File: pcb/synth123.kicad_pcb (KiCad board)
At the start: 2 copper layers, 100 x 50 mm, 29 parts, among them IC1 ATTINY4313, IC2 PC817, IC3 DAC, K1 STEREO/MONO, P1 POWER, P2 MIDI_IN, P3 ISP, P4 AUDIO_OUT, U1 7805, X1 20MHz

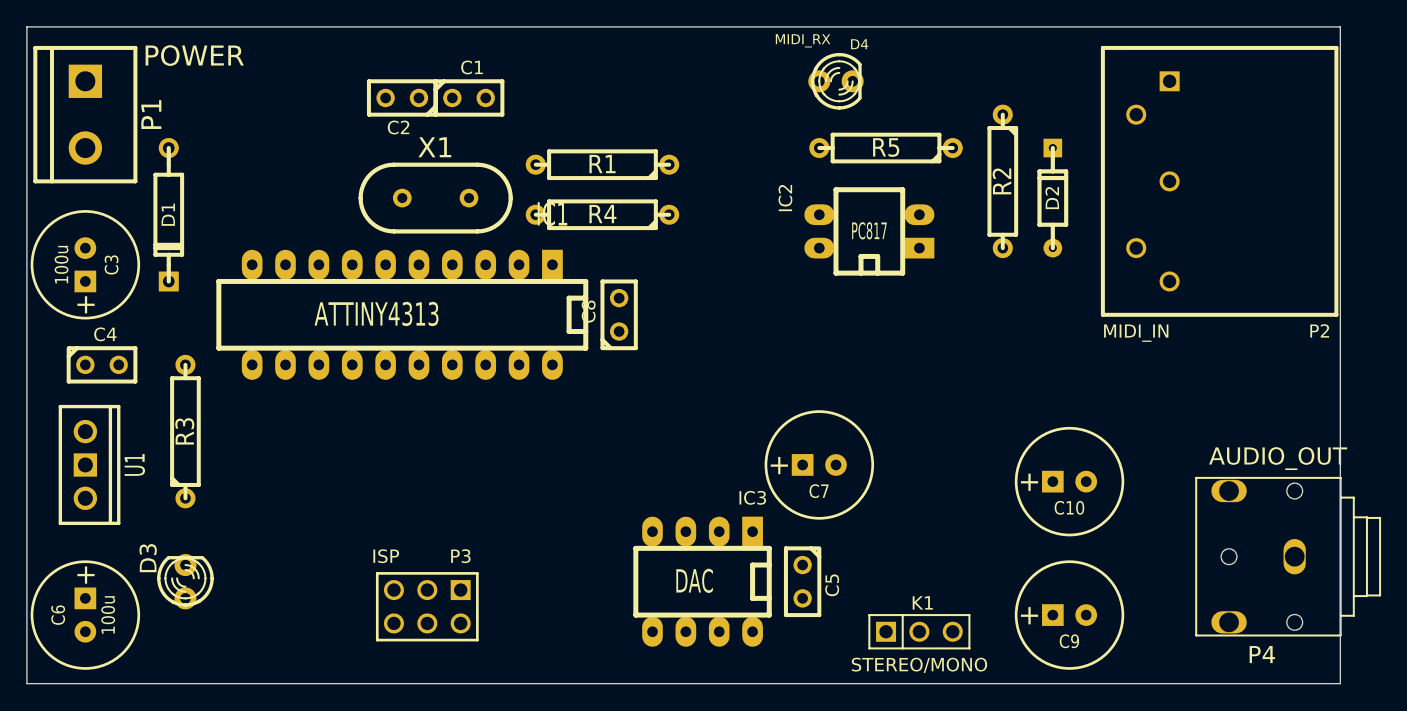
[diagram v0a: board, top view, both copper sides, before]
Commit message: Updated KiCad files.
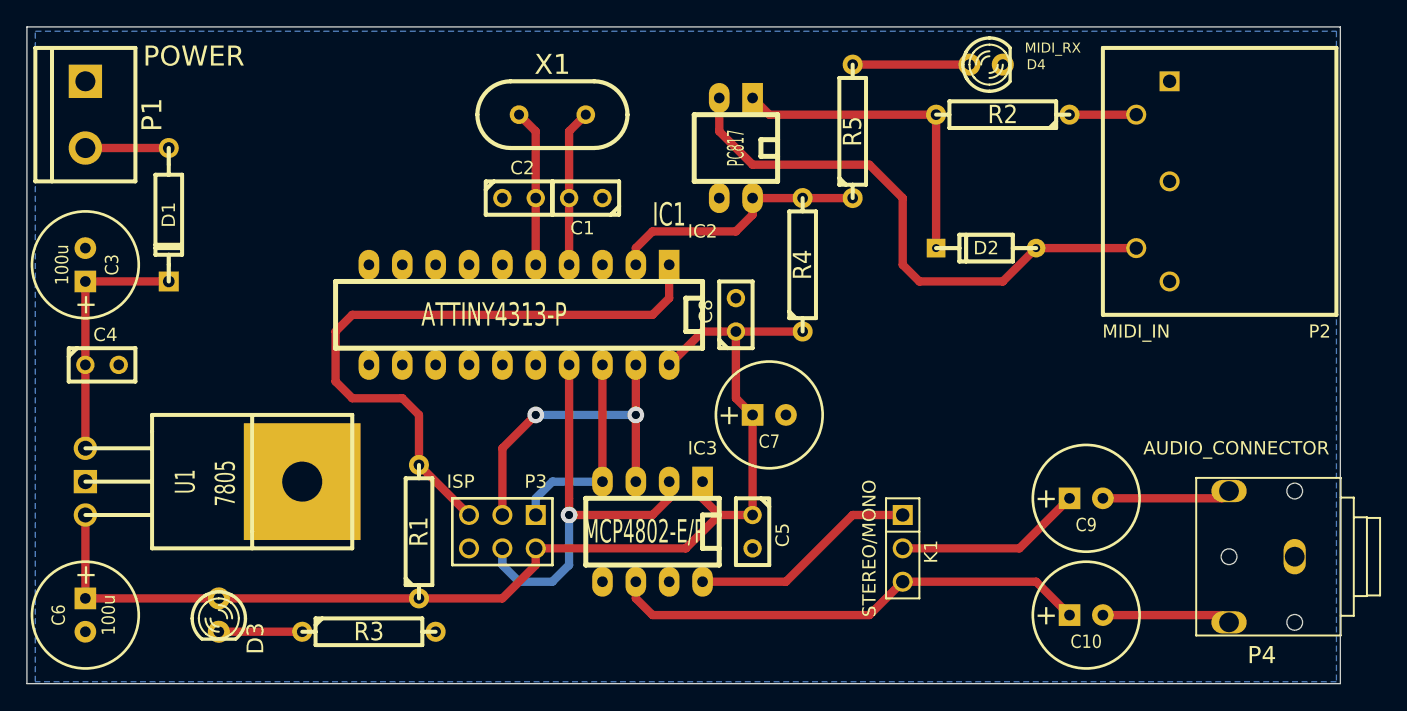
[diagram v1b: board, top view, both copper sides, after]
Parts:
- IC1: value ATTINY4313 -> ATTINY4313-P
- IC3: value DAC -> MCP4802-E/P
- P4: value AUDIO_OUT -> AUDIO_CONNECTOR
- U1: footprint LM78XXV -> LM78XX
- moved R1 31.2 mm to (92.7, 69.8), turned to 90 degrees
- moved R3 20.7 mm to (88.9, 77.5), turned to 0 degrees
- moved R4 15.7 mm to (121.9, 49.5), turned to 90 degrees
- moved IC2 12.0 mm to (116.8, 40.6), turned to 180 degrees
- moved C1 11.7 mm to (105.4, 44.5), turned to 180 degrees
- moved C2 11.7 mm to (100.3, 44.5), turned to 0 degrees
- moved D4 11.5 mm to (135.9, 34.3)
- moved X1 10.9 mm to (102.9, 38.1)
- moved C10 10.2 mm to (143.5, 76.2)
- moved C9 8.98 mm to (143.5, 67.3)
- moved C8 8.89 mm to (116.8, 53.3)
- moved IC1 8.89 mm to (100.3, 53.3)
- moved P3 8.08 mm to (99.1, 69.8)
- moved K1 6.48 mm to (129.5, 71.1), turned to 270 degrees
- moved D2 6.35 mm to (135.9, 48.3), turned to 180 degrees
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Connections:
- C10 pad 2: N-000003 -> N-0000020
- C9 pad 2: N-000001 (its old number) -> N-0000019
- P4 pad 2: N-000003 -> N-0000019
- P4 pad 5: N-000001 (its old number) -> N-0000020
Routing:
- net VCC: track 0.00 -> 89.3 mm
- net //RESET: track 0.00 -> 49.4 mm
- net N-0000025: track 0.00 -> 43.1 mm
- net N-0000018: track 0.00 -> 36.9 mm
- net N-000001: track 0.00 -> 32.1 mm, vias 0 -> 1
- net N-0000021: track 0.00 -> 25.2 mm, vias 0 -> 2
- net N-000002: track 0.00 -> 24.7 mm
- net N-0000013: track 0.00 -> 20.1 mm
- net N-0000016: track 0.00 -> 19.0 mm
- net N-0000010: track 0.00 -> 17.3 mm
- net N-0000022: track 0.00 -> 15.8 mm
- net N-0000015: track 0.00 -> 14.3 mm
- net N-0000024: track 0.00 -> 12.0 mm
- net N-0000023: track 0.00 -> 12.0 mm
- net N-0000019: track 0.00 -> 9.83 mm
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- added copper zone on B.Cu, net GND
